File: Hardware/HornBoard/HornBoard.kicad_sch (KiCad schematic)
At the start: 17 parts, among them J1 Horn Ctl, J2 Conn_01x03, J3 Horn In, J4 Horn Out

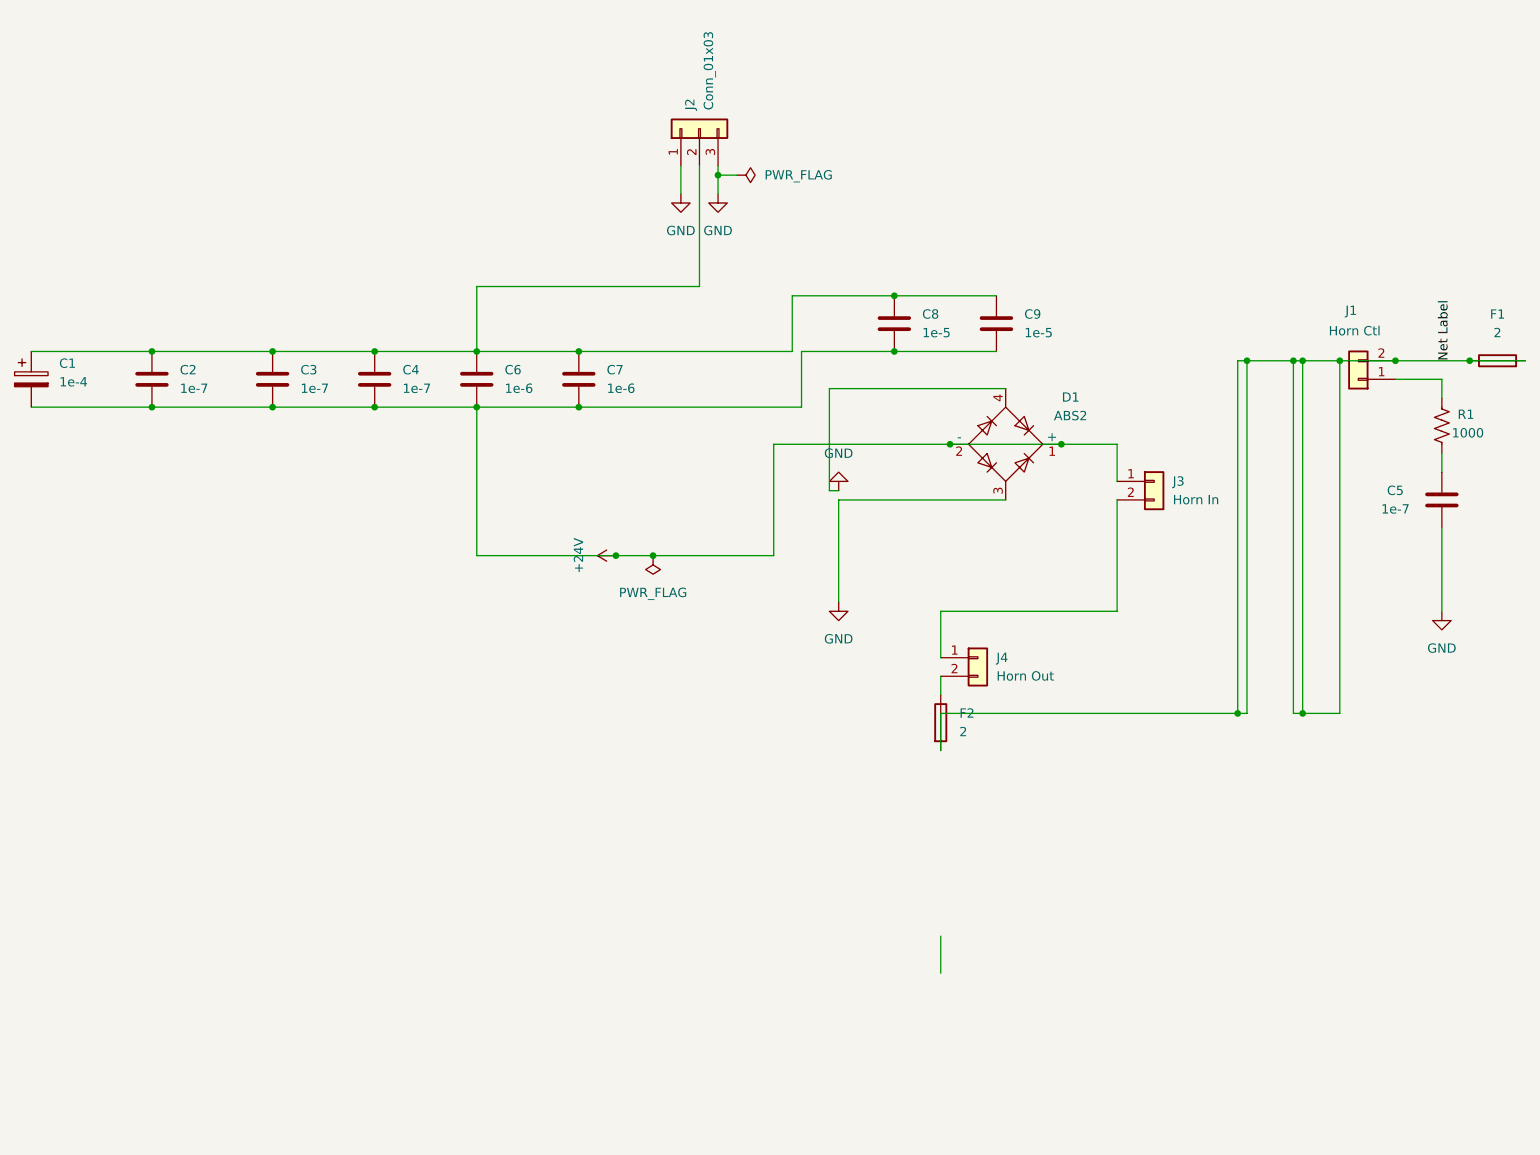
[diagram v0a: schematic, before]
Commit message: finish projects
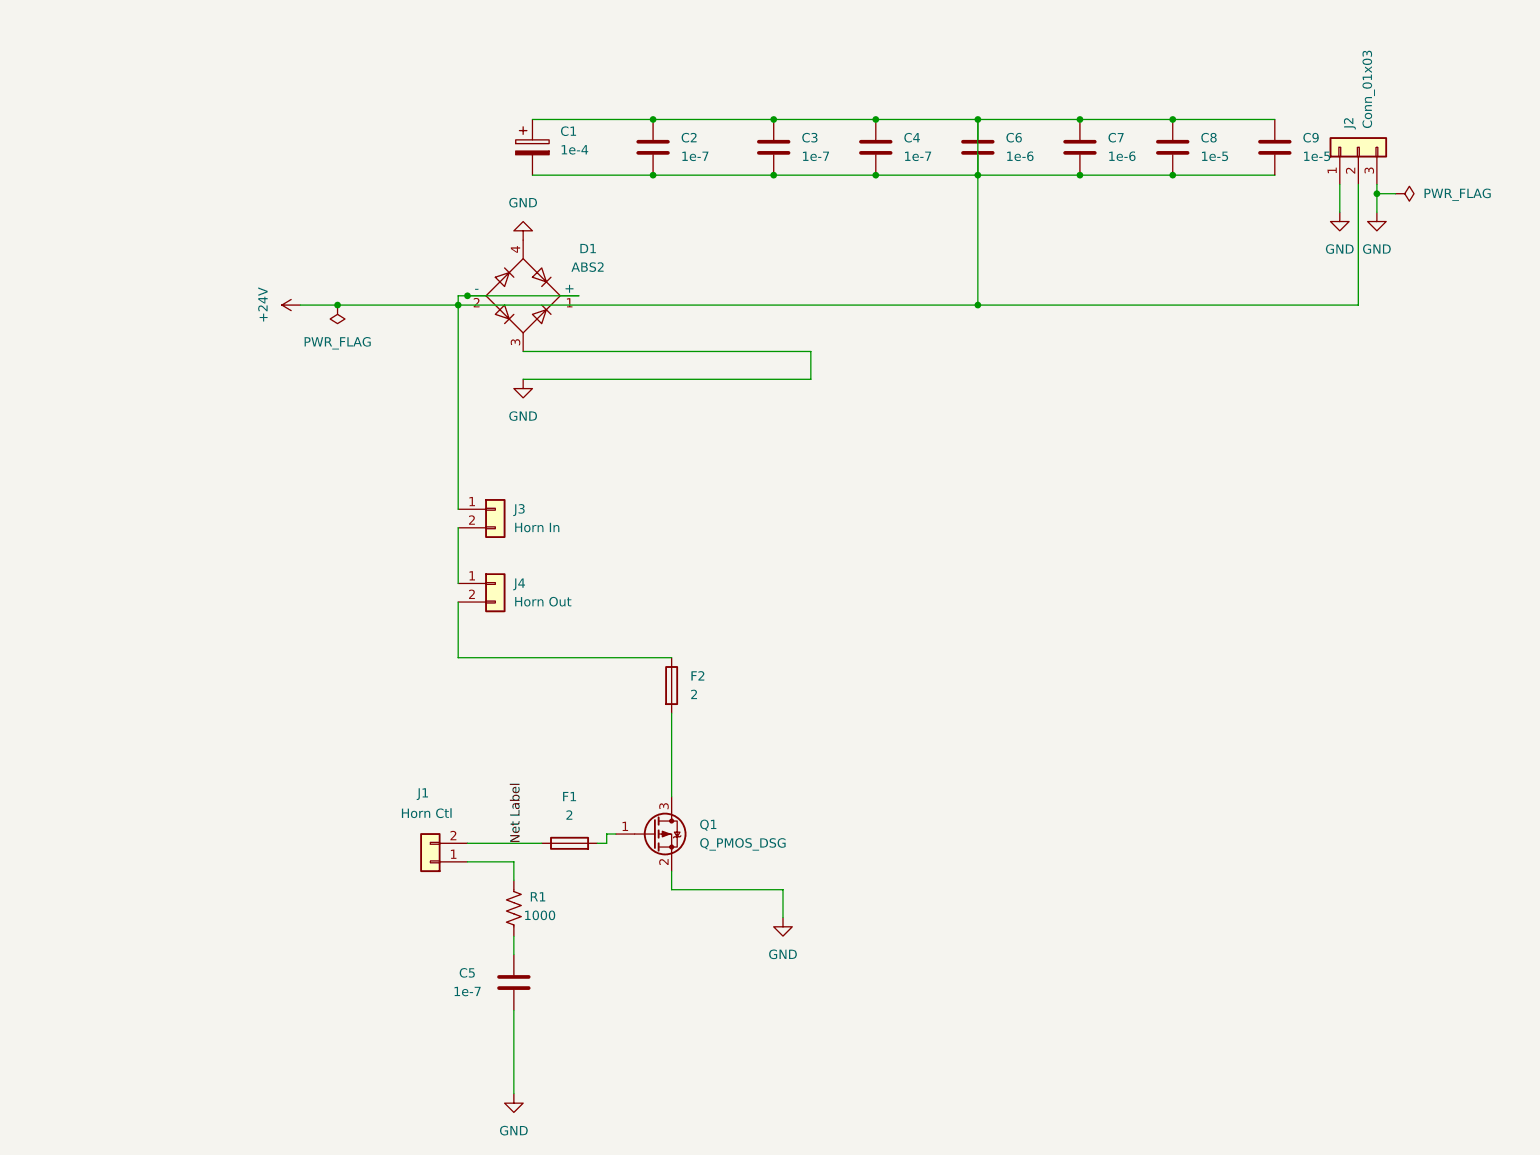
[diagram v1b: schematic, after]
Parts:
- added Q1: Q_PMOS_DSG, Package_TO_SOT_SMD:SOT-23, symbol device:Q_PMOS_GSD
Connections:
- net +24V: now also C1.1, C2.1, C3.1, C4.1, C6.1, C7.1, C8.1, C9.1, J2.2 (Pin_2)
- net GND: now also Q1.2 (S)
- net Net Label: no longer F1.2, F2.2
- new net: F1.2, Q1.1 (G)
- new net: F2.2, Q1.3 (D)
